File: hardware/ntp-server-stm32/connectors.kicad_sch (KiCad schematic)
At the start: 41 parts, among them J10 OSTVN02A150, J15 SMA-J-P-H-RA-TH1, J16 OSTVN06A150, J17 1787179, J2 OSTVN04A150, J3 BG055-06A-1-0450-0530-0350-L-D, J5 USB4120-03-C, J6 622-009-260-033, J7 SMA-J-P-H-RA-TH1, J8 SMA-J-P-H-RA-TH1, J9 SMA-J-P-H-RA-TH1, U15 TPD4E02B04DQAR, U16 TPD4E02B04DQAR, U17 TPD4E05U06DQAR, U18 TPD4E05U06DQAR, U19 TPD4E02B04DQAR, U20 TPD4E02B04DQAR, U65 TPD4E05U06DQAR, U66 TPD4E05U06DQAR, U69 TPD4E05U06DQAR, U70 TPD4E05U06DQAR

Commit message: Add files via upload
Updated, completed placement
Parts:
- C186, C42: footprint 1812 (4532 Metric) -> Capacitor_SMD:C_1812_4532Metric
- C188, C41, C43: footprint 0402 (1005 Metric) -> copy_ref:C_0402_1005Metric
- C40: footprint 0603 (1608 Metric) -> copy_ref:C_0603_1608Metric
- D22: footprint DO-219AB (SMF) -> dowload:DO-219AB (SMF)
- D23, D8, D9: footprint 2-XDFN -> dowload:2-XDFN
- D26: footprint DO-214AC -> dowload:DO-214AC
- D6: footprint DO-219AB (SMF) -> Diode_SMD:D_SMF
- D7: footprint DO-214AB (SMC) -> Diode_SMD:D_SMC
- J10: footprint (none) -> dowload:CONN_OSTVN02A150_OST
- J15, J7, J8, J9: footprint (none) -> dowload:SAMTEC_SMA-J-P-X-RA-TH1
- J16: footprint (none) -> dowload:CONN_OSTVN06A150_OST
- J17: footprint (none) -> dowload:PHOENIX_1787179
- J2: footprint (none) -> dowload:CONN_OSTVN04A150_OST
- J3: footprint Library:GCT_BG055-06A-1-0450-0530-0350-L-D -> dowload:GCT_BG055-06A-1-0450-0530-0350-L-D
- J6: footprint (none) -> copy_ref:DB9_Socket
- L10: footprint 0603 (1608 Metric) -> Inductor_SMD:L_0603_1608Metric
- R231, R64, R65, R66, R67, R68: footprint 0402 (1005 Metric) -> copy_ref:R_0402_1005Metric
- U15, U16, U17, U18, U19, U20: footprint 10-USON -> dowload:TPD4E02B04DQAR
- U65, U66, U69, U70: footprint 10-USON -> copy_ref:USON-10_2.5x1.0mm_P0.5mm
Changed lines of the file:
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@@
 			)
 		)
-		(property "Footprint" ""
+		(property "Footprint" "dowload:SAMTEC_SMA-J-P-X-RA-TH1"
 			(at 63.5 234.95 0)
 			(hide yes)
@@
 			)
 		)
-		(property "Footprint" "DO-214AC"
+		(property "Footprint" "dowload:DO-214AC"
 			(at 52.07 95.25 0)
 			(hide yes)
@@
 			)
 		)
-		(property "Footprint" "10-USON"
+		(property "Footprint" "dowload:TPD4E02B04DQAR"
 			(at 292.1 81.28 0)
 			(hide yes)
@@
 			)
 		)
-		(property "Footprint" "1812 (4532 Metric)"
+		(property "Footprint" "Capacitor_SMD:C_1812_4532Metric"
 			(at 102.5652 119.38 0)
 			(hide yes)
@@
 			)
 		)
-		(property "Footprint" ""
+		(property "Footprint" "dowload:SAMTEC_SMA-J-P-X-RA-TH1"
 			(at 63.5 201.93 0)
 			(hide yes)
@@
 			)
 		)
-		(property "Footprint" "2-XDFN"
+		(property "Footprint" "dowload:2-XDFN"
 			(at 57.15 254 0)
 			(hide yes)
@@
 			)
 		)
-		(property "Footprint" ""
+		(property "Footprint" "dowload:CONN_OSTVN06A150_OST"
 			(at 356.87 210.82 0)
 			(hide yes)
@@
 			)
 		)
-		(property "Footprint" "10-USON"
+		(property "Footprint" "copy_ref:USON-10_2.5x1.0mm_P0.5mm"
 			(at 292.1 125.73 0)
 			(hide yes)
@@
 			)
 		)
-		(property "Footprint" "0603 (1608 Metric)"
+		(property "Footprint" "Inductor_SMD:L_0603_1608Metric"
 			(at 49.53 218.44 0)
 			(hide yes)
@@
 			)
 		)
-		(property "Footprint" ""
+		(property "Footprint" "dowload:PHOENIX_1787179"
 			(at 172.72 217.17 0)
 			(hide yes)
@@
 			)
 		)
-		(property "Footprint" "10-USON"
+		(property "Footprint" "copy_ref:USON-10_2.5x1.0mm_P0.5mm"
 			(at 217.17 151.13 0)
 			(hide yes)
@@
 			)
 		)
-		(property "Footprint" "DO-219AB (SMF)"
+		(property "Footprint" "Diode_SMD:D_SMF"
 			(at 111.76 240.03 0)
 			(hide yes)
@@
 			)
 		)
-		(property "Footprint" "0402 (1005 Metric)"
+		(property "Footprint" "copy_ref:R_0402_1005Metric"
 			(at 163.83 24.638 90)
 			(hide yes)
@@
 			)
 		)
-		(property "Footprint" "0402 (1005 Metric)"
+		(property "Footprint" "copy_ref:R_0402_1005Metric"
 			(at 95.758 115.57 90)
 			(hide yes)
@@
 			)
 		)
-		(property "Footprint" "0402 (1005 Metric)"
+		(property "Footprint" "copy_ref:R_0402_1005Metric"
 			(at 141.478 69.85 90)
 			(hide yes)
@@
 			)
 		)
-		(property "Footprint" ""
+		(property "Footprint" "dowload:CONN_OSTVN02A150_OST"
 			(at 265.43 236.22 0)
 			(hide yes)
@@
 			)
 		)
-		(property "Footprint" "DO-214AB (SMC)"
+		(property "Footprint" "Diode_SMD:D_SMC"
 			(at 76.2 80.01 0)
 			(hide yes)
@@
 			)
 		)
-		(property "Footprint" "10-USON"
+		(property "Footprint" "copy_ref:USON-10_2.5x1.0mm_P0.5mm"
 			(at 292.1 171.45 0)
 			(hide yes)
@@
 			)
 		)
-		(property "Footprint" "0603 (1608 Metric)"
+		(property "Footprint" "copy_ref:C_0603_1608Metric"
 			(at 118.4148 243.84 0)
 			(hide yes)
@@
 			)
 		)
-		(property "Footprint" "0402 (1005 Metric)"
+		(property "Footprint" "copy_ref:R_0402_1005Metric"
 			(at 173.228 29.21 90)
 			(hide yes)
@@
 			)
 		)
-		(property "Footprint" ""
+		(property "Footprint" "copy_ref:DB9_Socket"
 			(at 93.98 88.9 0)
 			(hide yes)
@@
 			)
 		)
-		(property "Footprint" "0402 (1005 Metric)"
+		(property "Footprint" "copy_ref:C_0402_1005Metric"
 			(at 219.4052 228.6 0)
 			(hide yes)
@@
 			)
 		)
-		(property "Footprint" ""
+		(property "Footprint" "dowload:CONN_OSTVN04A150_OST"
 			(at 76.2 36.83 0)
 			(hide yes)
@@
 			)
 		)
-		(property "Footprint" "2-XDFN"
+		(property "Footprint" "dowload:2-XDFN"
 			(at 57.15 190.5 0)
 			(hide yes)
@@
 			)
 		)
-		(property "Footprint" "10-USON"
+		(property "Footprint" "dowload:TPD4E02B04DQAR"
 			(at 374.65 125.73 0)
 			(hide yes)
@@
 			)
 		)
-		(property "Footprint" "10-USON"
+		(property "Footprint" "copy_ref:USON-10_2.5x1.0mm_P0.5mm"
 			(at 374.65 40.64 0)
 			(hide yes)
@@
 			)
 		)
-		(property "Footprint" "0402 (1005 Metric)"
+		(property "Footprint" "copy_ref:R_0402_1005Metric"
 			(at 205.232 78.74 90)
 			(hide yes)
@@
 			)
 		)
-		(property "Footprint" "10-USON"
+		(property "Footprint" "dowload:TPD4E02B04DQAR"
 			(at 374.65 171.45 0)
 			(hide yes)
@@
 			)
 		)
-		(property "Footprint" "10-USON"
+		(property "Footprint" "dowload:TPD4E02B04DQAR"
 			(at 153.67 151.13 0)
 			(hide yes)
@@
 			)
 		)
-		(property "Footprint" "0402 (1005 Metric)"
+		(property "Footprint" "copy_ref:R_0402_1005Metric"
 			(at 150.368 104.14 90)
 			(hide yes)
@@
 			)
 		)
-		(property "Footprint" "2-XDFN"
+		(property "Footprint" "dowload:2-XDFN"
 			(at 57.15 165.1 0)
 			(hide yes)
@@
 			)
 		)
-		(property "Footprint" "10-USON"
+		(property "Footprint" "dowload:TPD4E02B04DQAR"
 			(at 374.65 81.28 0)
 			(hide yes)
@@
 			)
 		)
-		(property "Footprint" "0402 (1005 Metric)"
+		(property "Footprint" "copy_ref:C_0402_1005Metric"
 			(at 126.6952 243.84 0)
 			(hide yes)
@@
 			)
 		)
-		(property "Footprint" ""
+		(property "Footprint" "dowload:SAMTEC_SMA-J-P-X-RA-TH1"
 			(at 63.5 171.45 0)
 			(hide yes)
@@
 			)
 		)
-		(property "Footprint" ""
+		(property "Footprint" "dowload:SAMTEC_SMA-J-P-X-RA-TH1"
 			(at 63.5 146.05 0)
 			(hide yes)
@@
 			)
 		)
-		(property "Footprint" "Library:GCT_BG055-06A-1-0450-0530-0350-L-D"
+		(property "Footprint" "dowload:GCT_BG055-06A-1-0450-0530-0350-L-D"
 			(at 27.94 40.64 0)
 			(hide yes)
@@
 			)
 		)
-		(property "Footprint" "0402 (1005 Metric)"
+		(property "Footprint" "copy_ref:C_0402_1005Metric"
 			(at 182.5752 33.02 0)
 			(hide yes)
@@
 			)
 		)
-		(property "Footprint" "10-USON"
+		(property "Footprint" "dowload:TPD4E02B04DQAR"
 			(at 290.83 40.64 0)
 			(hide yes)
@@
 			)
 		)
-		(property "Footprint" "DO-219AB (SMF)"
+		(property "Footprint" "dowload:DO-219AB (SMF)"
 			(at 217.17 224.79 0)
 			(hide yes)
@@
 			)
 		)
-		(property "Footprint" "1812 (4532 Metric)"
+		(property "Footprint" "Capacitor_SMD:C_1812_4532Metric"
 			(at 157.1752 107.95 0)
 			(hide yes)

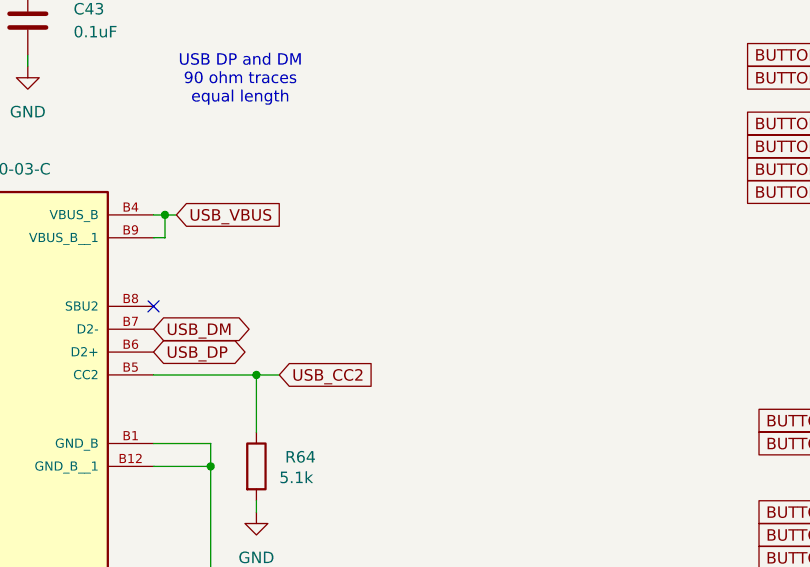
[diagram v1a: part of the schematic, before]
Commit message: PCB / 3D updates
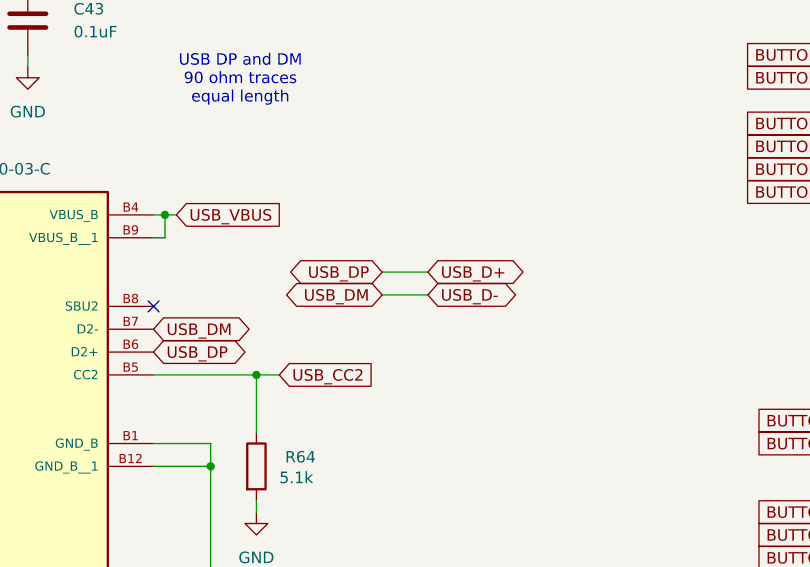
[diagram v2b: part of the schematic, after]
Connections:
- net USB_DM renamed USB_D-
- net USB_DP renamed USB_D+
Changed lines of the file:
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@@
 	(wire
 		(pts
+			(xy 220.98 57.15) (xy 226.06 57.15)
+		)
+		(stroke
+			(width 0)
+			(type default)
+		)
+	)
+	(wire
+		(pts
 			(xy 160.02 53.34) (xy 158.75 53.34)
 		)
@@
 	(wire
 		(pts
+			(xy 220.98 59.69) (xy 226.06 59.69)
+		)
+		(stroke
+			(width 0)
+			(type default)
+		)
+	)
+	(wire
+		(pts
 			(xy 392.43 45.72) (xy 394.97 45.72)
 		)
@@
 		)
 	)
+	(global_label "USB_D+"
+		(shape bidirectional)
+		(at 226.06 57.15 0)
+		(fields_autoplaced yes)
+		(effects
+			(font
+				(size 1.27 1.27)
+			)
+			(justify left)
+		)
+		(property "Intersheetrefs" "${INTERSHEET_REFS}"
+			(at 237.7765 57.15 0)
+			(hide yes)
+			(show_name no)
+			(do_not_autoplace no)
+			(effects
+				(font
+					(size 1.27 1.27)
+				)
+				(justify left)
+			)
+		)
+	)
 	(global_label "BUTTON_3"
 		(shape input)
@@
 		)
 	)
+	(global_label "USB_DP"
+		(shape bidirectional)
+		(at 220.98 57.15 180)
+		(fields_autoplaced yes)
+		(effects
+			(font
+				(size 1.27 1.27)
+			)
+			(justify right)
+		)
+		(property "Intersheetrefs" "${INTERSHEET_REFS}"
+			(at 209.5659 57.15 0)
+			(hide yes)
+			(show_name no)
+			(do_not_autoplace no)
+			(effects
+				(font
+					(size 1.27 1.27)
+				)
+				(justify right)
+			)
+		)
+	)
 	(global_label "PANEL_LED_WHITE_N_4"
 		(shape input)
@@
 		)
 	)
+	(global_label "USB_DM"
+		(shape bidirectional)
+		(at 220.98 59.69 180)
+		(fields_autoplaced yes)
+		(effects
+			(font
+				(size 1.27 1.27)
+			)
+			(justify right)
+		)
+		(property "Intersheetrefs" "${INTERSHEET_REFS}"
+			(at 209.3845 59.69 0)
+			(hide yes)
+			(show_name no)
+			(do_not_autoplace no)
+			(effects
+				(font
+					(size 1.27 1.27)
+				)
+				(justify right)
+			)
+		)
+	)
 	(global_label "USB_DP"
 		(shape bidirectional)
@@
 			)
 		)
+	)
+	(global_label "USB_D-"
+		(shape bidirectional)
+		(at 226.06 59.69 0)
+		(fields_autoplaced yes)
+		(effects
+			(font
+				(size 1.27 1.27)
+			)
+			(justify left)
+		)
+		(property "Intersheetrefs" "${INTERSHEET_REFS}"
+			(at 237.7765 59.69 0)
+			(hide yes)
+			(show_name no)
+			(do_not_autoplace no)
+			(effects
+				(font
+					(size 1.27 1.27)
+				)
+				(justify left)
+			)
+		)
